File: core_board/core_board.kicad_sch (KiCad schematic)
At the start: 16 parts

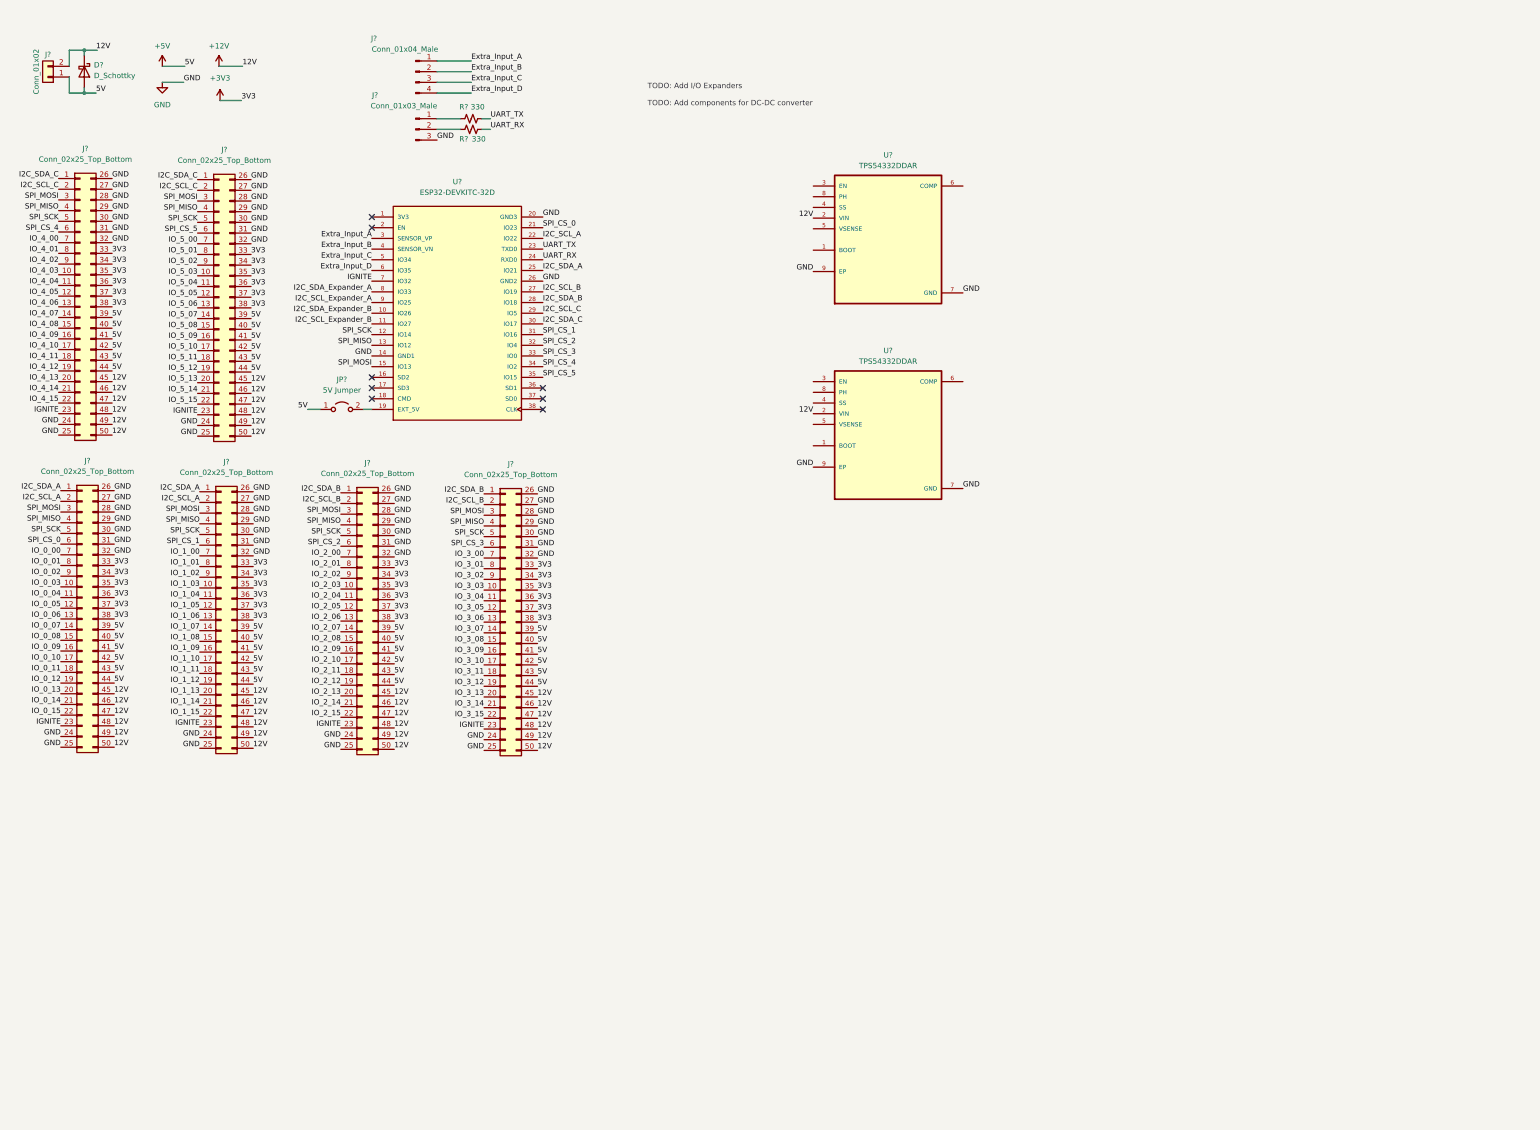
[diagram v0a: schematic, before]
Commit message: small updates
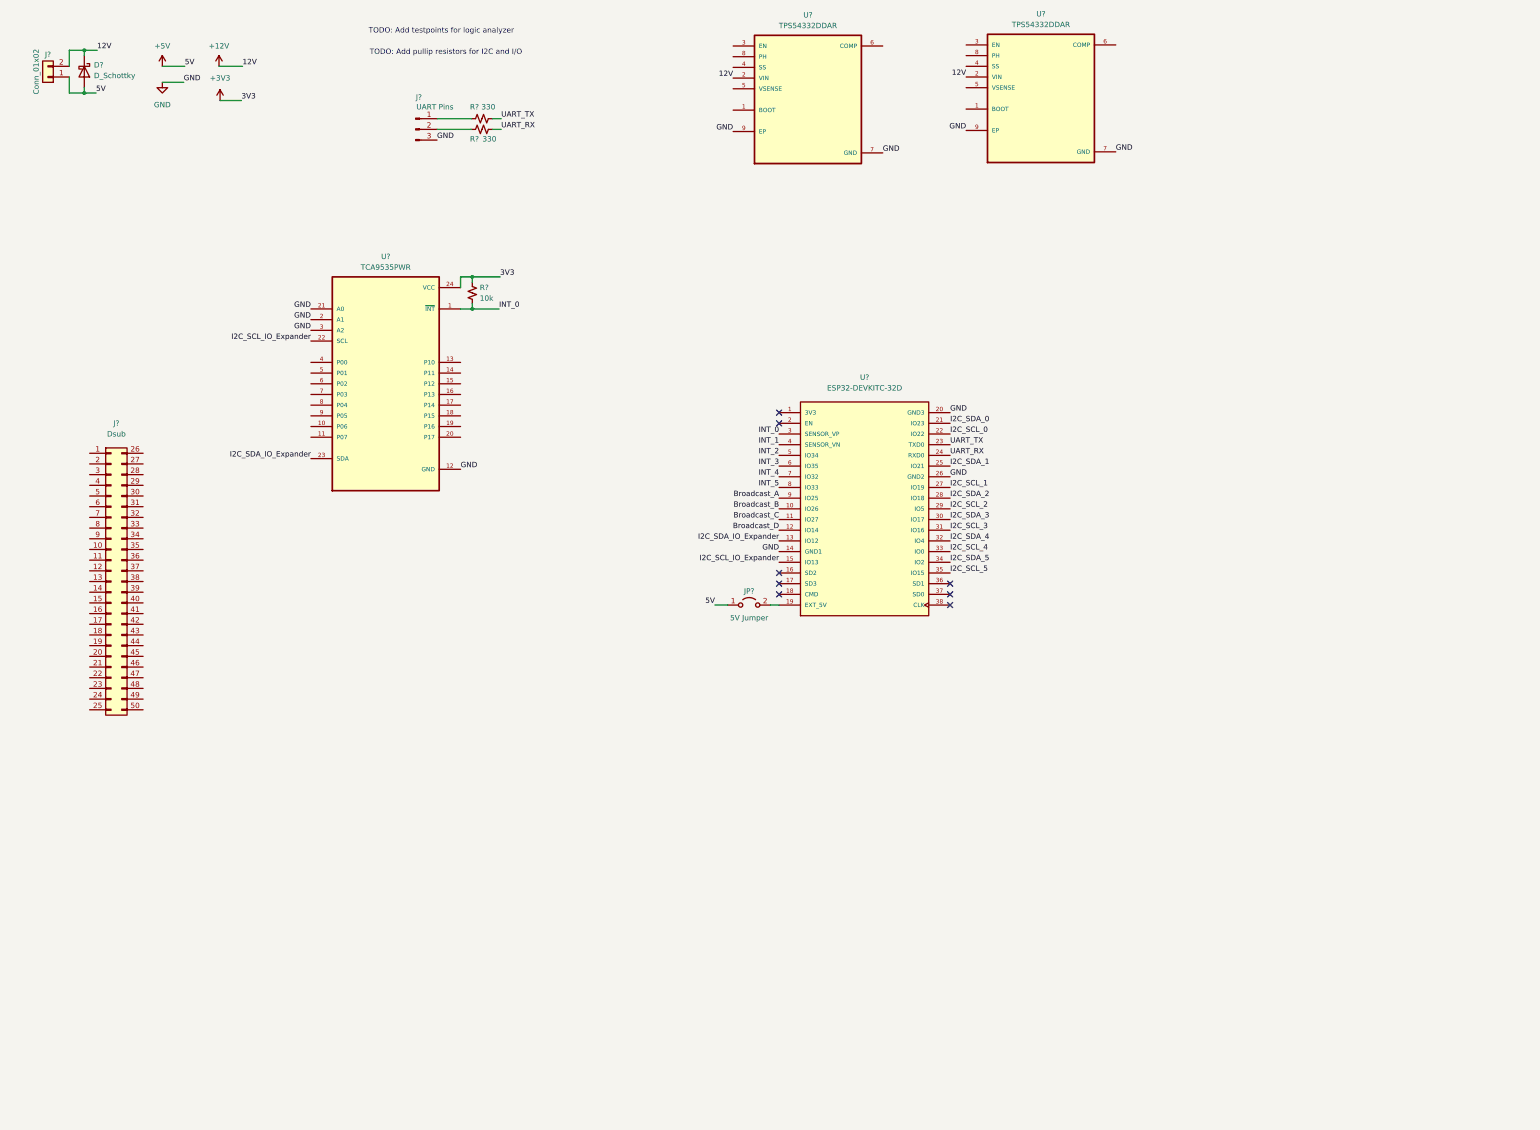
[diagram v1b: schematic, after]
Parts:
- removed J?: Conn_01x04_Male, symbol Connector:Conn_01x04_Male
- removed J? (x6): Conn_02x25_Top_Bottom, symbol Connector_Generic:Conn_02x25_Top_Bottom
- added J?: Dsub, symbol Connector_Generic:Conn_02x25_Top_Bottom
- added R?: 10k, symbol Device:R_Small_US
- added U?: TCA9535PWR, SOP65P640X120-24N, symbol TCA9535PWR:TCA9535PWR
- J?: value Conn_01x03_Male -> UART Pins
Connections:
- net +3V3: now also R?.1, U?.24 (VCC)
- net GND: now also U?.12 (GND), U?.2 (A1), U?.21 (A0), U?.3 (A2)
- net Extra_Input_A renamed INT_0
- net INT_0: now also R?.2, U?.1 (~{INT})
- net Extra_Input_B renamed INT_1
- net Extra_Input_C renamed INT_2
- net Extra_Input_D renamed INT_3
- net I2C_SCL_A renamed I2C_SCL_0
- net I2C_SCL_B renamed I2C_SCL_1
- net I2C_SCL_C renamed I2C_SCL_2
- net I2C_SCL_Expander_A renamed Broadcast_A
- net I2C_SCL_Expander_B renamed Broadcast_C
- net I2C_SDA_A renamed I2C_SDA_1
- net I2C_SDA_B renamed I2C_SDA_2
- net I2C_SDA_C renamed I2C_SDA_3
- net I2C_SDA_Expander_A renamed INT_5
- net I2C_SDA_Expander_B renamed Broadcast_B
- net IGNITE renamed INT_4
- net SPI_CS_0 renamed I2C_SDA_0
- net SPI_CS_1 renamed I2C_SCL_3
- net SPI_CS_2 renamed I2C_SDA_4
- net SPI_CS_3 renamed I2C_SCL_4
- net SPI_CS_4 renamed I2C_SDA_5
- net SPI_CS_5 renamed I2C_SCL_5
- net SPI_MISO renamed I2C_SDA_IO_Expander
- net I2C_SDA_IO_Expander: now also U?.23 (SDA)
- net SPI_MOSI renamed I2C_SCL_IO_Expander
- net I2C_SCL_IO_Expander: now also U?.22 (SCL)
- net SPI_SCK renamed Broadcast_D
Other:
- note added: "TODO: Add pullip resistors for I2C and I/O"
- note added: "TODO: Add testpoints for logic analyzer"
- note removed: "TODO: Add I/O Expanders"
- note removed: "TODO: Add components for DC-DC converter"
- moved on the sheet: JP?, R?, U?

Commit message: finished schematic
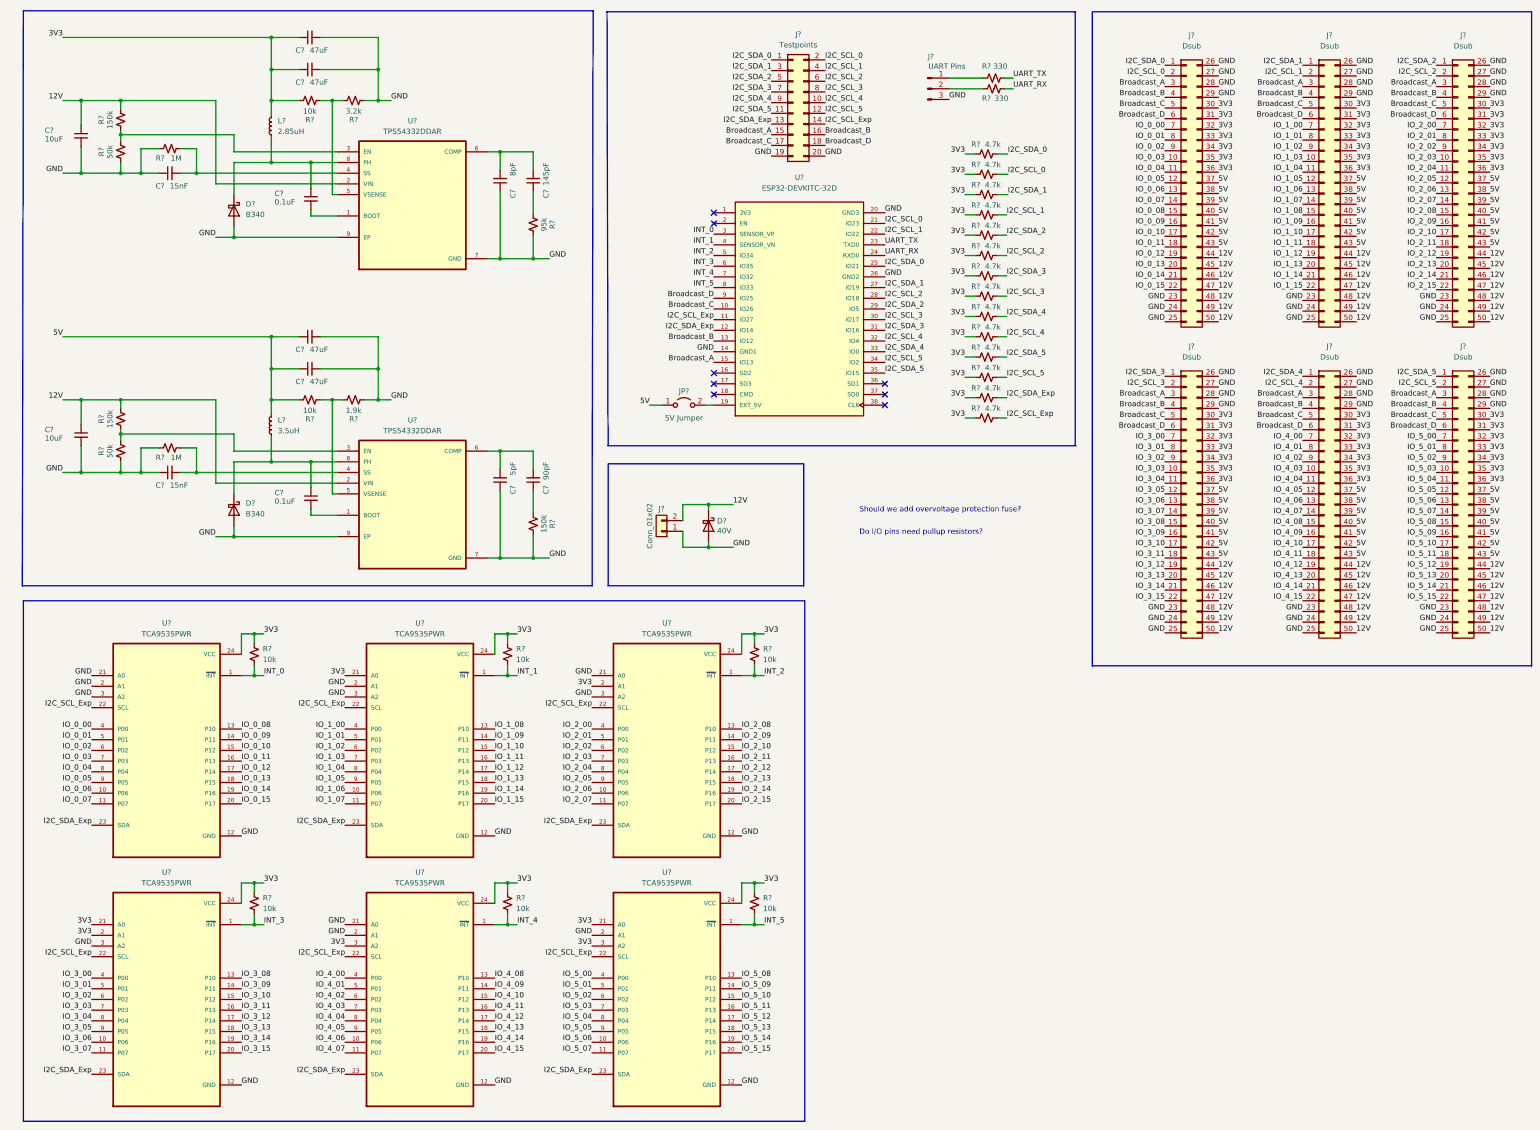
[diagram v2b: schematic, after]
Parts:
- removed D?: D_Schottky, symbol Device:D_Schottky
- removed R?: 10k, symbol Device:R_Small_US
- removed U?: TPS54332DDAR, VREG_LM5017MR/NOPB, symbol TPS54332DDAR:TPS54332DDAR
- added C? (x2): 10uF, symbol Device:C_Small
- added C? (x4): 47uF, symbol Device:C_Small
- added C?: 145pF, symbol Device:C_Small
- added C?: 90pF, symbol Device:C_Small
- added C?: 5pF, symbol Device:C_Small
- added C?: 8pF, symbol Device:C_Small
- added C? (x2): 15nF, symbol Device:C_Small
- added C? (x2): 0.1uF, symbol Device:C_Small
- added D? (x2): B340, Diode_SMD:D_SMC, symbol Diode:B340
- added D?: 40V, Diode_SMD:D_0603_1608Metric, symbol Device:D_Schottky
- added J? (x5): Dsub, symbol Connector_Generic:Conn_02x25_Top_Bottom
- added J?: Testpoints, symbol Connector_Generic:Conn_02x10_Odd_Even
- added L?: 2.85uH, symbol Device:L_Small
- added L?: 3.5uH, symbol Device:L_Small
- added R? (x14): 4.7k, symbol Device:R_Small_US
- added R? (x3): 150k, symbol Device:R_Small_US
- added R? (x8): 10k, symbol Device:R_Small_US
- added R? (x2): 1M, symbol Device:R_Small_US
- added R?: 3.2k, symbol Device:R_Small_US
- added R?: 95k, symbol Device:R_Small_US
- added R? (x2): 50k, symbol Device:R_Small_US
- added R?: 1.9k, symbol Device:R_Small_US
- added U? (x5): TCA9535PWR, SOP65P640X120-24N, symbol TCA9535PWR:TCA9535PWR
- added U?: TPS54332DDAR, VREG_LM5017MR/NOPB, symbol TPS54332DDAR:TPS54332DDAR
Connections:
- net +12V is gone; now on net 12V: J?.2 (Pin_2), U?.2 (VIN)
- net +3V3 is gone; now on net 3V3: U?.24 (VCC)
- net Broadcast_A: now also J?.3 (Pin_3), U?.15 (IO13), J?.15 (Pin_15), J?.3 (Pin_3), J?.3 (Pin_3), J?.3 (Pin_3), J?.3 (Pin_3), J?.3 (Pin_3); no longer U?.9 (IO25)
- net Broadcast_B: now also J?.4 (Pin_4), U?.13 (IO12), J?.16 (Pin_16), J?.4 (Pin_4), J?.4 (Pin_4), J?.4 (Pin_4), J?.4 (Pin_4), J?.4 (Pin_4); no longer U?.10 (IO26)
- net Broadcast_C: now also J?.5 (Pin_5), U?.10 (IO26), J?.17 (Pin_17), J?.5 (Pin_5), J?.5 (Pin_5), J?.5 (Pin_5), J?.5 (Pin_5), J?.5 (Pin_5); no longer U?.11 (IO27)
- net Broadcast_D: now also J?.6 (Pin_6), U?.9 (IO25), J?.18 (Pin_18), J?.6 (Pin_6), J?.6 (Pin_6), J?.6 (Pin_6), J?.6 (Pin_6), J?.6 (Pin_6); no longer U?.12 (IO14)
- net GND: now also J?.1 (Pin_1), J?.23 (Pin_23), J?.24 (Pin_24), J?.25 (Pin_25), J?.26 (Pin_26), J?.27 (Pin_27), J?.28 (Pin_28), J?.29 (Pin_29), C?.1, C?.1, C?.1, C?.1, C?.2, C?.2, C?.2, C?.2, C?.2, C?.2, D?.2 (A), D?.2 (A), D?.2 (A), J?.19 (Pin_19), J?.20 (Pin_20), J?.23 (Pin_23), J?.23 (Pin_23), J?.23 (Pin_23), J?.23 (Pin_23), J?.23 (Pin_23), J?.24 (Pin_24), J?.24 (Pin_24), J?.24 (Pin_24), J?.24 (Pin_24), J?.24 (Pin_24), J?.25 (Pin_25), J?.25 (Pin_25), J?.25 (Pin_25), J?.25 (Pin_25), J?.25 (Pin_25), J?.26 (Pin_26), J?.26 (Pin_26), J?.26 (Pin_26), J?.26 (Pin_26), J?.26 (Pin_26), J?.27 (Pin_27), J?.27 (Pin_27), J?.27 (Pin_27), J?.27 (Pin_27), J?.27 (Pin_27), J?.28 (Pin_28), J?.28 (Pin_28), J?.28 (Pin_28), J?.28 (Pin_28), J?.28 (Pin_28), J?.29 (Pin_29), J?.29 (Pin_29), J?.29 (Pin_29), J?.29 (Pin_29), J?.29 (Pin_29), R?.1, R?.1, R?.1, R?.1, R?.1, R?.1, R?.2, R?.2, U?.12 (GND), U?.12 (GND), U?.12 (GND), U?.12 (GND), U?.12 (GND), U?.2 (A1), U?.2 (A1), U?.2 (A1), U?.2 (A1), U?.21 (A0), U?.21 (A0), U?.21 (A0), U?.3 (A2), U?.3 (A2), U?.3 (A2), U?.7 (GND), U?.9 (EP); no longer U?.2 (A1), U?.21 (A0)
- net I2C_SCL_0: now also U?.21 (IO23), J?.2 (Pin_2), J?.2 (Pin_2), R?.2; no longer U?.22 (IO22)
- net I2C_SCL_1: now also U?.22 (IO22), J?.2 (Pin_2), J?.4 (Pin_4), R?.2; no longer U?.27 (IO19)
- net I2C_SCL_2: now also U?.28 (IO18), J?.2 (Pin_2), J?.6 (Pin_6), R?.2; no longer U?.29 (IO5)
- net I2C_SCL_3: now also J?.2 (Pin_2), U?.30 (IO17), J?.8 (Pin_8), R?.2; no longer U?.31 (IO16)
- net I2C_SCL_4: now also U?.32 (IO4), J?.10 (Pin_10), J?.2 (Pin_2), R?.2; no longer U?.33 (IO0)
- net I2C_SCL_5: now also U?.34 (IO2), J?.12 (Pin_12), J?.2 (Pin_2), R?.2; no longer U?.35 (IO15)
- net I2C_SDA_0: now also U?.25 (IO21), J?.1 (Pin_1), J?.1 (Pin_1), R?.2; no longer U?.21 (IO23)
- net I2C_SDA_1: now also U?.27 (IO19), J?.1 (Pin_1), J?.3 (Pin_3), R?.2; no longer U?.25 (IO21)
- net I2C_SDA_2: now also U?.29 (IO5), J?.1 (Pin_1), J?.5 (Pin_5), R?.2; no longer U?.28 (IO18)
- net I2C_SDA_3: now also J?.1 (Pin_1), U?.31 (IO16), J?.7 (Pin_7), R?.2; no longer U?.30 (IO17)
- net I2C_SDA_4: now also U?.33 (IO0), J?.1 (Pin_1), J?.9 (Pin_9), R?.2; no longer U?.32 (IO4)
- net I2C_SDA_5: now also U?.35 (IO15), J?.1 (Pin_1), J?.11 (Pin_11), R?.2; no longer U?.34 (IO2)
- net INT_0: now also R?.2, U?.1 (~{INT}); no longer U?.1 (~{INT})
- net INT_1: now also R?.2, U?.1 (~{INT})
- net INT_2: now also R?.2, U?.1 (~{INT})
- net INT_3: now also U?.1 (~{INT}), R?.2
- net INT_4: now also R?.2, U?.1 (~{INT})
- net INT_5: now also R?.2, U?.1 (~{INT})
- net IO_3_06: now reaches U?.10 (P06)
- net IO_3_06: now also J?.13 (Pin_13)
- net IO_3_07: now reaches U?.11 (P07)
- net IO_3_07: now also J?.14 (Pin_14)
- net IO_3_08: now reaches U?.13 (P10)
- net IO_3_08: now also J?.15 (Pin_15)
- net IO_3_09: now reaches U?.14 (P11)
- net IO_3_09: now also J?.16 (Pin_16)
- net IO_3_10: now reaches U?.15 (P12)
- net IO_3_10: now also J?.17 (Pin_17)
- net IO_3_11: now reaches U?.16 (P13)
- net IO_3_11: now also J?.18 (Pin_18)
- net IO_3_12: now reaches U?.17 (P14)
- net IO_3_12: now also J?.19 (Pin_19)
- net IO_3_13: now reaches U?.18 (P15)
- net IO_3_13: now also J?.20 (Pin_20)
- net IO_3_14: now reaches U?.19 (P16)
- net IO_3_14: now also J?.21 (Pin_21)
- net IO_3_15: now reaches U?.20 (P17)
- net IO_3_15: now also J?.22 (Pin_22)
- net IO_3_00: now reaches U?.4 (P00)
- net IO_3_00: now also J?.7 (Pin_7)
- net IO_3_01: now reaches U?.5 (P01)
- net IO_3_01: now also J?.8 (Pin_8)
- net IO_3_02: now reaches U?.6 (P02)
- net IO_3_02: now also J?.9 (Pin_9)
- net IO_3_03: now reaches U?.7 (P03)
- net IO_3_03: now also J?.10 (Pin_10)
- net IO_3_04: now reaches U?.8 (P04)
- net IO_3_04: now also J?.11 (Pin_11)
- net IO_3_05: now reaches U?.9 (P05)
- net IO_3_05: now also J?.12 (Pin_12)
- net at U?.1 (BOOT): now also C?.2
- net at U?.3 (EN): now also R?.1, R?.2
- net at U?.4 (SS): now also C?.2, R?.2
- net at U?.5 (VSENSE): now also R?.1, R?.2
- net at U?.6 (COMP): now also C?.2, C?.2
- net at U?.8 (PH): now also C?.1, D?.1 (K), L?.1
- net 3V3: now reaches J?.30 (Pin_30)
- net 3V3: now also J?.31 (Pin_31), J?.32 (Pin_32), J?.33 (Pin_33), J?.34 (Pin_34), J?.35 (Pin_35), J?.36 (Pin_36), U?.2 (A1), U?.21 (A0), C?.1, C?.1, J?.30 (Pin_30), J?.30 (Pin_30), J?.30 (Pin_30), J?.30 (Pin_30), J?.30 (Pin_30), J?.31 (Pin_31), J?.31 (Pin_31), J?.31 (Pin_31), J?.31 (Pin_31), J?.31 (Pin_31), J?.32 (Pin_32), J?.32 (Pin_32), J?.32 (Pin_32), J?.32 (Pin_32), J?.32 (Pin_32), J?.33 (Pin_33), J?.33 (Pin_33), J?.33 (Pin_33), J?.33 (Pin_33), J?.33 (Pin_33), J?.34 (Pin_34), J?.34 (Pin_34), J?.34 (Pin_34), J?.34 (Pin_34), J?.34 (Pin_34), J?.35 (Pin_35), J?.35 (Pin_35), J?.35 (Pin_35), J?.35 (Pin_35), J?.35 (Pin_35), J?.36 (Pin_36), J?.36 (Pin_36), J?.36 (Pin_36), J?.36 (Pin_36), J?.36 (Pin_36), L?.2, R?.1, R?.1, R?.1, R?.1, R?.1, R?.1, R?.1, R?.1, R?.1, R?.1, R?.1, R?.1, R?.1, R?.1, R?.1, R?.1, R?.1, R?.1, R?.1, R?.1, R?.2, U?.2 (A1), U?.21 (A0), U?.21 (A0), U?.24 (VCC), U?.24 (VCC), U?.24 (VCC), U?.24 (VCC), U?.24 (VCC), U?.3 (A2), U?.3 (A2)
- net 5V: now reaches J?.37 (Pin_37)
- net 5V: now also J?.38 (Pin_38), J?.39 (Pin_39), J?.40 (Pin_40), J?.41 (Pin_41), J?.42 (Pin_42), J?.43 (Pin_43), JP?.1 (A), C?.1, C?.1, J?.37 (Pin_37), J?.37 (Pin_37), J?.37 (Pin_37), J?.37 (Pin_37), J?.37 (Pin_37), J?.38 (Pin_38), J?.38 (Pin_38), J?.38 (Pin_38), J?.38 (Pin_38), J?.38 (Pin_38), J?.39 (Pin_39), J?.39 (Pin_39), J?.39 (Pin_39), J?.39 (Pin_39), J?.39 (Pin_39), J?.40 (Pin_40), J?.40 (Pin_40), J?.40 (Pin_40), J?.40 (Pin_40), J?.40 (Pin_40), J?.41 (Pin_41), J?.41 (Pin_41), J?.41 (Pin_41), J?.41 (Pin_41), J?.41 (Pin_41), J?.42 (Pin_42), J?.42 (Pin_42), J?.42 (Pin_42), J?.42 (Pin_42), J?.42 (Pin_42), J?.43 (Pin_43), J?.43 (Pin_43), J?.43 (Pin_43), J?.43 (Pin_43), J?.43 (Pin_43), L?.2, R?.2
- net 12V: now reaches J?.44 (Pin_44)
- net 12V: now also J?.45 (Pin_45), J?.46 (Pin_46), J?.47 (Pin_47), J?.48 (Pin_48), J?.49 (Pin_49), J?.50 (Pin_50), C?.1, C?.1, D?.1 (K), J?.44 (Pin_44), J?.44 (Pin_44), J?.44 (Pin_44), J?.44 (Pin_44), J?.44 (Pin_44), J?.45 (Pin_45), J?.45 (Pin_45), J?.45 (Pin_45), J?.45 (Pin_45), J?.45 (Pin_45), J?.46 (Pin_46), J?.46 (Pin_46), J?.46 (Pin_46), J?.46 (Pin_46), J?.46 (Pin_46), J?.47 (Pin_47), J?.47 (Pin_47), J?.47 (Pin_47), J?.47 (Pin_47), J?.47 (Pin_47), J?.48 (Pin_48), J?.48 (Pin_48), J?.48 (Pin_48), J?.48 (Pin_48), J?.48 (Pin_48), J?.49 (Pin_49), J?.49 (Pin_49), J?.49 (Pin_49), J?.49 (Pin_49), J?.49 (Pin_49), J?.50 (Pin_50), J?.50 (Pin_50), J?.50 (Pin_50), J?.50 (Pin_50), J?.50 (Pin_50), R?.2, R?.2, U?.2 (VIN)
- removed net +5V: J?.1 (Pin_1), JP?.1 (A)
- net I2C_SCL_IO_Expander renamed I2C_SCL_Exp
- net I2C_SCL_Exp: now also U?.11 (IO27), J?.14 (Pin_14), R?.2, U?.22 (SCL), U?.22 (SCL), U?.22 (SCL), U?.22 (SCL), U?.22 (SCL); no longer U?.15 (IO13)
- net I2C_SDA_IO_Expander renamed I2C_SDA_Exp
- net I2C_SDA_Exp: now also U?.12 (IO14), J?.13 (Pin_13), R?.2, U?.23 (SDA), U?.23 (SDA), U?.23 (SDA), U?.23 (SDA), U?.23 (SDA); no longer U?.13 (IO12)
- new net: C?.1, D?.1 (K), L?.1, U?.8 (PH)
- new net: R?.1, R?.2, U?.3 (EN)
- new net: R?.1, R?.2, U?.5 (VSENSE)
- new net: C?.1, R?.1 (x2)
- new net: C?.2, R?.2, U?.4 (SS)
- new net: C?.2, C?.2, U?.6 (COMP)
- new net: C?.2, U?.1 (BOOT)
- new net IO_0_00: J?.7 (Pin_7), U?.4 (P00)
- new net IO_0_01: J?.8 (Pin_8), U?.5 (P01)
- new net IO_0_02: J?.9 (Pin_9), U?.6 (P02)
- new net IO_0_03: J?.10 (Pin_10), U?.7 (P03)
- new net IO_0_04: J?.11 (Pin_11), U?.8 (P04)
- new net IO_0_05: J?.12 (Pin_12), U?.9 (P05)
- new net IO_0_06: J?.13 (Pin_13), U?.10 (P06)
- new net IO_0_07: J?.14 (Pin_14), U?.11 (P07)
- new net IO_0_08: J?.15 (Pin_15), U?.13 (P10)
- new net IO_0_09: J?.16 (Pin_16), U?.14 (P11)
- new net IO_0_10: J?.17 (Pin_17), U?.15 (P12)
- new net IO_0_11: J?.18 (Pin_18), U?.16 (P13)
- new net IO_0_12: J?.19 (Pin_19), U?.17 (P14)
- new net IO_0_13: J?.20 (Pin_20), U?.18 (P15)
- new net IO_0_14: J?.21 (Pin_21), U?.19 (P16)
- new net IO_0_15: J?.22 (Pin_22), U?.20 (P17)
- new net IO_1_00: J?.7 (Pin_7), U?.4 (P00)
- new net IO_1_01: J?.8 (Pin_8), U?.5 (P01)
- new net IO_1_02: J?.9 (Pin_9), U?.6 (P02)
- new net IO_1_03: J?.10 (Pin_10), U?.7 (P03)
- new net IO_1_04: J?.11 (Pin_11), U?.8 (P04)
- new net IO_1_05: J?.12 (Pin_12), U?.9 (P05)
- new net IO_1_06: J?.13 (Pin_13), U?.10 (P06)
- new net IO_1_07: J?.14 (Pin_14), U?.11 (P07)
- new net IO_1_08: J?.15 (Pin_15), U?.13 (P10)
- new net IO_1_09: J?.16 (Pin_16), U?.14 (P11)
- new net IO_1_10: J?.17 (Pin_17), U?.15 (P12)
- new net IO_1_11: J?.18 (Pin_18), U?.16 (P13)
- new net IO_1_12: J?.19 (Pin_19), U?.17 (P14)
- new net IO_1_13: J?.20 (Pin_20), U?.18 (P15)
- new net IO_1_14: J?.21 (Pin_21), U?.19 (P16)
- new net IO_1_15: J?.22 (Pin_22), U?.20 (P17)
- new net IO_2_00: J?.7 (Pin_7), U?.4 (P00)
- new net IO_2_01: J?.8 (Pin_8), U?.5 (P01)
- new net IO_2_02: J?.9 (Pin_9), U?.6 (P02)
- new net IO_2_03: J?.10 (Pin_10), U?.7 (P03)
- new net IO_2_04: J?.11 (Pin_11), U?.8 (P04)
- new net IO_2_05: J?.12 (Pin_12), U?.9 (P05)
- new net IO_2_06: J?.13 (Pin_13), U?.10 (P06)
- new net IO_2_07: J?.14 (Pin_14), U?.11 (P07)
- new net IO_2_08: J?.15 (Pin_15), U?.13 (P10)
- new net IO_2_09: J?.16 (Pin_16), U?.14 (P11)
- new net IO_2_10: J?.17 (Pin_17), U?.15 (P12)
- new net IO_2_11: J?.18 (Pin_18), U?.16 (P13)
- new net IO_2_12: J?.19 (Pin_19), U?.17 (P14)
- new net IO_2_13: J?.20 (Pin_20), U?.18 (P15)
- new net IO_2_14: J?.21 (Pin_21), U?.19 (P16)
- new net IO_2_15: J?.22 (Pin_22), U?.20 (P17)
- new net IO_4_00: J?.7 (Pin_7), U?.4 (P00)
- new net IO_4_01: J?.8 (Pin_8), U?.5 (P01)
- new net IO_4_02: J?.9 (Pin_9), U?.6 (P02)
- new net IO_4_03: J?.10 (Pin_10), U?.7 (P03)
- new net IO_4_04: J?.11 (Pin_11), U?.8 (P04)
- new net IO_4_05: J?.12 (Pin_12), U?.9 (P05)
- new net IO_4_06: J?.13 (Pin_13), U?.10 (P06)
- new net IO_4_07: J?.14 (Pin_14), U?.11 (P07)
- new net IO_4_08: J?.15 (Pin_15), U?.13 (P10)
- new net IO_4_09: J?.16 (Pin_16), U?.14 (P11)
- new net IO_4_10: J?.17 (Pin_17), U?.15 (P12)
- new net IO_4_11: J?.18 (Pin_18), U?.16 (P13)
- new net IO_4_12: J?.19 (Pin_19), U?.17 (P14)
- new net IO_4_13: J?.20 (Pin_20), U?.18 (P15)
- new net IO_4_14: J?.21 (Pin_21), U?.19 (P16)
- new net IO_4_15: J?.22 (Pin_22), U?.20 (P17)
- new net IO_5_00: J?.7 (Pin_7), U?.4 (P00)
- new net IO_5_01: J?.8 (Pin_8), U?.5 (P01)
- new net IO_5_02: J?.9 (Pin_9), U?.6 (P02)
- new net IO_5_03: J?.10 (Pin_10), U?.7 (P03)
- new net IO_5_04: J?.11 (Pin_11), U?.8 (P04)
- new net IO_5_05: J?.12 (Pin_12), U?.9 (P05)
- new net IO_5_06: J?.13 (Pin_13), U?.10 (P06)
- new net IO_5_07: J?.14 (Pin_14), U?.11 (P07)
- new net IO_5_08: J?.15 (Pin_15), U?.13 (P10)
- new net IO_5_09: J?.16 (Pin_16), U?.14 (P11)
- new net IO_5_10: J?.17 (Pin_17), U?.15 (P12)
- new net IO_5_11: J?.18 (Pin_18), U?.16 (P13)
- new net IO_5_12: J?.19 (Pin_19), U?.17 (P14)
- new net IO_5_13: J?.20 (Pin_20), U?.18 (P15)
- new net IO_5_14: J?.21 (Pin_21), U?.19 (P16)
- new net IO_5_15: J?.22 (Pin_22), U?.20 (P17)
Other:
- note added: "Do I/O pins need pullup resistors?"
- note added: "Should we add overvoltage protection fuse?"
- note removed: "TODO: Add pullip resistors for I2C and I/O"
- note removed: "TODO: Add testpoints for logic analyzer"
- moved on the sheet: J?, JP?, R?, U?
